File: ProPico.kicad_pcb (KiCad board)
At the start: 2 copper layers, 21 x 51 mm, 55 parts, among them J1 USB_C_Receptacle_USB2.0, J2 SWD, J3 LEFT, J4 RIGHT, SW1 BOOTSEL, SW2 RES, U1 FM24CL16B, U2 W25Q128JVS, U3 TLV1117-33, U4 LM4040DBZ-3, U5 RP2040, Y1 ECS-120-12-36-AGN-TR3

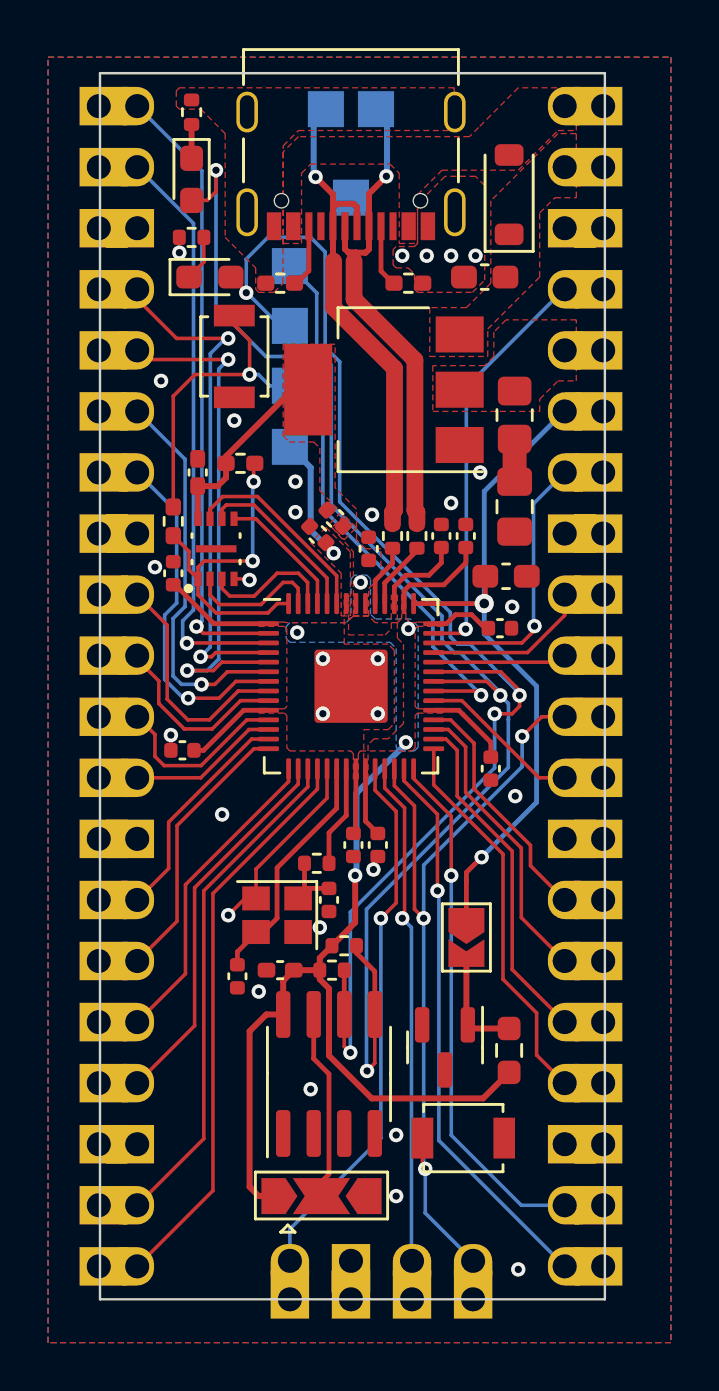
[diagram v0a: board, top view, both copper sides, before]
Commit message: finished erc
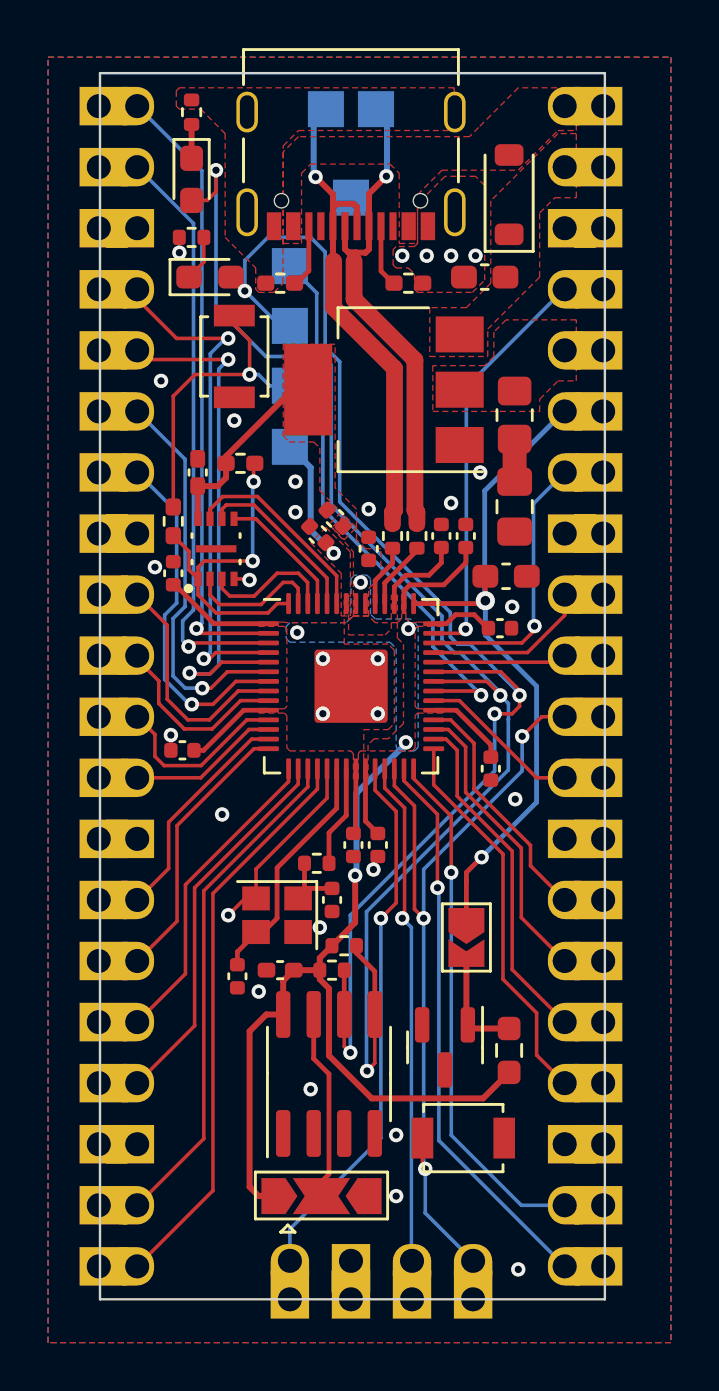
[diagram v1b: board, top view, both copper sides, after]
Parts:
- moved C3 0.13 mm to (154.1, 83.3)
